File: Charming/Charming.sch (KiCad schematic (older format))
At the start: 98 parts, among them J1 Conn_02x12_Odd_Even, SW1 SW_Push, SW10 SW_Push, SW11 SW_Push, SW12 SW_Push, SW13 SW_Push, SW14 SW_Push, SW15 SW_Push, SW16 SW_Push, SW17 SW_Push, SW18 SW_Push, SW19 SW_Push, SW2 SW_Push, SW20 SW_Push, SW21 SW_Push, SW22 SW_Push, SW23 SW_Push, SW24 SW_Push, SW25 SW_Push, SW26 SW_Push, SW27 SW_Push, SW28 SW_Push, SW29 SW_Push, SW3 SW_Push, SW30 SW_Push, SW31 SW_Push, SW32 SW_Push, SW33 SW_Push, SW34 SW_Push, SW35 SW_Push, SW36 SW_Push, SW37 SW_Push, SW38 SW_Push, SW39 SW_Push, SW4 SW_Push, SW40 SW_Push, SW41 SW_Push, SW42 SW_Push, SW43 SW_Push, SW44 SW_Push, SW45 SW_Push, SW46 SW_Push, SW47 SW_Push, SW48 SW_Push, SW5 SW_Push, SW6 SW_Push, SW7 SW_Push, SW8 SW_Push, SW9 SW_Push, U1 ProMicro

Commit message: nice and clean signal lines
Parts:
- removed J1: Conn_02x12_Odd_Even, Connector_PinSocket_2.54mm:PinSocket_2x12_P2.54mm_Vertical, symbol Connector_Generic:Conn_02x12_Odd_Even
- D1: symbol Device:D -> Diode:1N4148W
- U1: footprint Connector_PinSocket_2.54mm:PinSocket_2x12_P2.54mm_Vertical -> Keebio:ArduinoProMicro
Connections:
- wire segments 121 -> 113
- no-connect marks 8 -> 4
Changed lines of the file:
@@
 Text GLabel 2200 2350 0    50   Input ~ 0
 row3
-Text GLabel 2200 2150 0    50   Input ~ 0
+Text GLabel 3600 2350 2    50   Input ~ 0
 col6
-Text GLabel 2200 2050 0    50   Input ~ 0
+Text GLabel 3600 2250 2    50   Input ~ 0
 col7
-Text GLabel 2200 1950 0    50   Input ~ 0
+Text GLabel 3600 2050 2    50   Input ~ 0
 col8
-Text GLabel 2200 1850 0    50   Input ~ 0
+Text GLabel 3600 1950 2    50   Input ~ 0
 col9
-Text GLabel 2200 1750 0    50   Input ~ 0
+Text GLabel 3600 1850 2    50   Input ~ 0
 col10
-Text GLabel 2200 1650 0    50   Input ~ 0
+Text GLabel 3600 1750 2    50   Input ~ 0
 col11
 NoConn ~ 3600 1450
@@
 	1850 3800 1850 4500
 $Comp
-L Device:D D1
+L Diode:1N4148W D1
 U 1 1 5EEA2409
 P 2250 3950
 F 0 "D1" V 2296 3870 50  0000 R CNN
-F 1 "D" V 2205 3870 50  0000 R CNN
+F 1 "D" V 2205 3870 50  0001 R CNN
 F 2 "Diode_SMD:D_SOD-123" H 2250 3950 50  0001 C CNN
 F 3 "~" H 2250 3950 50  0001 C CNN
@@
 	1    0    0    -1
 $EndComp
-Text GLabel 2200 2250 0    50   Input ~ 0
-row2
 $Comp
 L keebio:ProMicro U1
@@
 F 0 "U1" H 2900 2637 60  0000 C CNN
 F 1 "ProMicro" H 2900 2531 60  0000 C CNN
-F 2 "Connector_PinSocket_2.54mm:PinSocket_2x12_P2.54mm_Vertical" H 3950 -700 60  0001 C CNN
+F 2 "Keebio:ArduinoProMicro" H 3950 -700 60  0001 C CNN
 F 3 "" V 3950 -700 60  0001 C CNN
 	1    2900 1800
 	1    0    0    -1
 $EndComp
-Wire Wire Line
-	5750 1600 5350 1600
-$Comp
-L power:GND #PWR0101
-U 1 1 5EF07202
-P 5900 1650
-F 0 "#PWR0101" H 5900 1400 50  0001 C CNN
-F 1 "GND" H 5905 1477 50  0000 C CNN
-F 2 "" H 5900 1650 50  0001 C CNN
-F 3 "" H 5900 1650 50  0001 C CNN
-	1    5900 1650
-	1    0    0    -1
-$EndComp
-Wire Wire Line
-	5900 1400 5900 1650
-Wire Wire Line
-	5750 1350 5750 1600
-$Comp
-L power:VCC #PWR0102
-U 1 1 5EF0720A
-P 5750 1350
-F 0 "#PWR0102" H 5750 1200 50  0001 C CNN
-F 1 "VCC" H 5765 1523 50  0000 C CNN
-F 2 "" H 5750 1350 50  0001 C CNN
-F 3 "" H 5750 1350 50  0001 C CNN
-	1    5750 1350
-	1    0    0    -1
-$EndComp
-Wire Wire Line
-	5350 1400 5900 1400
-$Comp
-L power:GND #PWR0103
-U 1 1 5EF0E795
-P 4400 1800
-F 0 "#PWR0103" H 4400 1550 50  0001 C CNN
-F 1 "GND" H 4405 1627 50  0000 C CNN
-F 2 "" H 4400 1800 50  0001 C CNN
-F 3 "" H 4400 1800 50  0001 C CNN
-	1    4400 1800
-	1    0    0    -1
-$EndComp
-Wire Wire Line
-	4850 1500 4400 1500
-Wire Wire Line
-	4850 1600 4400 1600
-Wire Wire Line
-	4400 1500 4400 1600
-Wire Wire Line
-	4400 1600 4400 1800
-Connection ~ 4400 1600
-NoConn ~ 5350 1300
-NoConn ~ 5350 1500
-NoConn ~ 4850 1400
-NoConn ~ 4850 1300
-$Comp
-L Connector_Generic:Conn_02x12_Odd_Even J1
-U 1 1 5EF52355
-P 5050 1800
-F 0 "J1" H 5100 2517 50  0000 C CNN
-F 1 "Conn_02x12_Odd_Even" H 5100 2426 50  0000 C CNN
-F 2 "Connector_PinSocket_2.54mm:PinSocket_2x12_P2.54mm_Vertical" H 5050 1800 50  0001 C CNN
-F 3 "~" H 5050 1800 50  0001 C CNN
-	1    5050 1800
-	1    0    0    -1
-$EndComp
-Text GLabel 3600 2350 2    50   Input ~ 0
+Text GLabel 2200 2150 0    50   Input ~ 0
 col5
-Text GLabel 3600 2250 2    50   Input ~ 0
+Text GLabel 2200 2050 0    50   Input ~ 0
 col4
+Text GLabel 2200 1950 0    50   Input ~ 0
+col3
+Text GLabel 2200 1850 0    50   Input ~ 0
+col2
+Text GLabel 2200 1650 0    50   Input ~ 0
+col0
 Text GLabel 3600 2150 2    50   Input ~ 0
-col3
-Text GLabel 3600 2050 2    50   Input ~ 0
-col2
-Text GLabel 3600 1850 2    50   Input ~ 0
-col0
-Text GLabel 3600 1750 2    50   Input ~ 0
 row1
-Text GLabel 3600 1950 2    50   Input ~ 0
+Text GLabel 2200 1750 0    50   Input ~ 0
 col1
 Wire Wire Line
@@
 Wire Wire Line
 	4000 1550 3600 1550
-Text GLabel 5350 2400 2    50   Input ~ 0
-col3
-Text GLabel 5350 2300 2    50   Input ~ 0
-col2
-Text GLabel 5350 2100 2    50   Input ~ 0
-col0
-Text GLabel 5350 2200 2    50   Input ~ 0
-col1
-Text GLabel 5350 1900 2    50   Input ~ 0
+Text GLabel 2200 2250 0    50   Input ~ 0
 row2
-Text GLabel 5350 2000 2    50   Input ~ 0
-row3
-Text GLabel 5350 1800 2    50   Input ~ 0
-row1
-Text GLabel 5350 1700 2    50   Input ~ 0
-row0
-Text GLabel 4850 2200 0    50   Input ~ 0
-col6
-Text GLabel 4850 2100 0    50   Input ~ 0
-col7
-Text GLabel 4850 2000 0    50   Input ~ 0
-col8
-Text GLabel 4850 1900 0    50   Input ~ 0
-col9
-Text GLabel 4850 1800 0    50   Input ~ 0
-col10
-Text GLabel 4850 1700 0    50   Input ~ 0
-col11
-Text GLabel 4850 2300 0    50   Input ~ 0
-col5
-Text GLabel 4850 2400 0    50   Input ~ 0
-col4
 $EndSCHEMATC

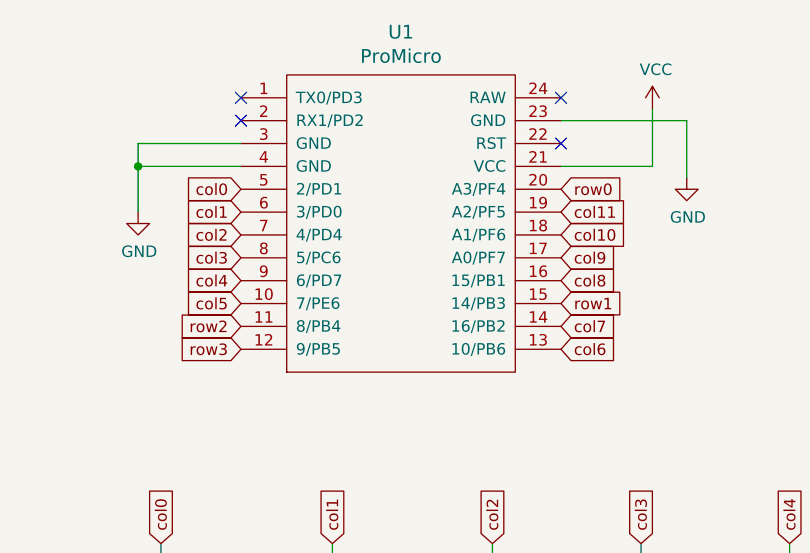
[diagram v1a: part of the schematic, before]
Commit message: v2
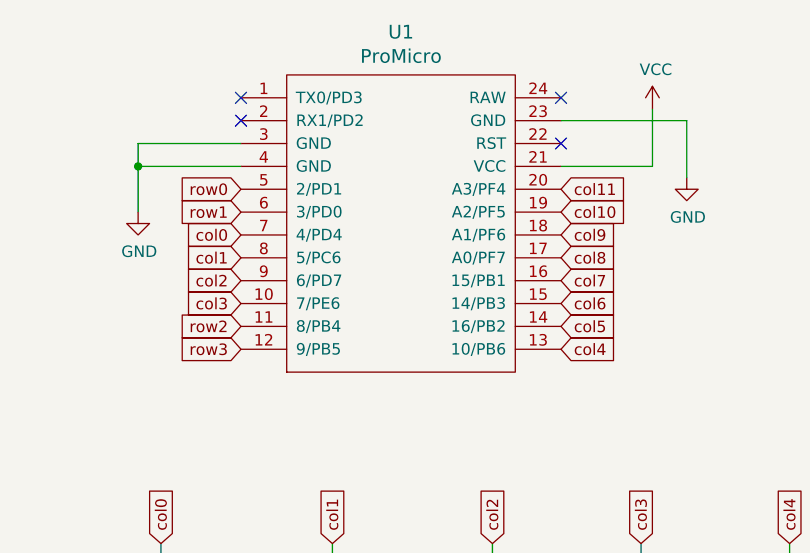
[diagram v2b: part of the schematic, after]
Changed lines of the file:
@@
 encoding utf-8
 Sheet 1 1
-Title "Charming"
-Date "2020-06-18"
-Rev "1.0"
+Title "Charming 40"
+Date "2020-06-21"
+Rev "2"
 Comp "Designed by James Sa"
 Comment1 ""
@@
 Text GLabel 2200 2350 0    50   Input ~ 0
 row3
-Text GLabel 3600 2350 2    50   Input ~ 0
+Text GLabel 3600 2150 2    50   Input ~ 0
 col6
-Text GLabel 3600 2250 2    50   Input ~ 0
+Text GLabel 3600 2050 2    50   Input ~ 0
 col7
-Text GLabel 3600 2050 2    50   Input ~ 0
+Text GLabel 3600 1950 2    50   Input ~ 0
 col8
-Text GLabel 3600 1950 2    50   Input ~ 0
+Text GLabel 3600 1850 2    50   Input ~ 0
 col9
-Text GLabel 3600 1850 2    50   Input ~ 0
+Text GLabel 3600 1750 2    50   Input ~ 0
 col10
-Text GLabel 3600 1750 2    50   Input ~ 0
+Text GLabel 3600 1650 2    50   Input ~ 0
 col11
 NoConn ~ 3600 1450
@@
 	1    0    0    -1
 $EndComp
+Text GLabel 3600 2250 2    50   Input ~ 0
+col5
+Text GLabel 3600 2350 2    50   Input ~ 0
+col4
 Text GLabel 2200 2150 0    50   Input ~ 0
-col5
+col3
 Text GLabel 2200 2050 0    50   Input ~ 0
-col4
+col2
+Text GLabel 2200 1850 0    50   Input ~ 0
+col0
+Text GLabel 2200 1750 0    50   Input ~ 0
+row1
 Text GLabel 2200 1950 0    50   Input ~ 0
-col3
-Text GLabel 2200 1850 0    50   Input ~ 0
-col2
+col1
+Wire Wire Line
+	3600 1350 4150 1350
 Text GLabel 2200 1650 0    50   Input ~ 0
-col0
-Text GLabel 3600 2150 2    50   Input ~ 0
-row1
-Text GLabel 2200 1750 0    50   Input ~ 0
-col1
-Wire Wire Line
-	3600 1350 4150 1350
-Text GLabel 3600 1650 2    50   Input ~ 0
 row0
 $Comp
